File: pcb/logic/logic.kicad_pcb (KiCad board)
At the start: 4 copper layers, 40.5 x 65 mm, 10 parts, among them J1 Conn_02x02_Odd_Even, J2 Conn_02x03_Odd_Even, J3 Conn_02x02_Odd_Even, J4 Conn_02x03_Odd_Even, J5 Conn_02x02_Odd_Even, J6 Conn_02x03_Odd_Even, U4 STM32G431C6Tx

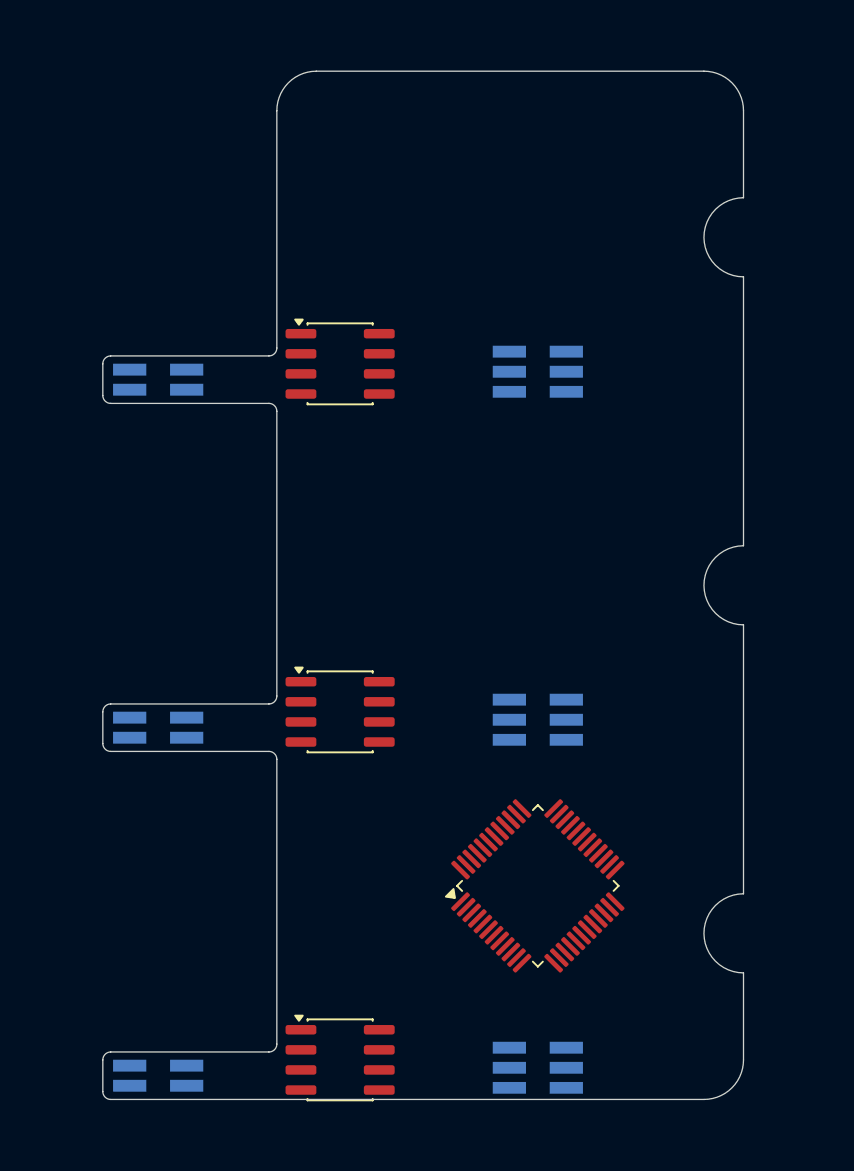
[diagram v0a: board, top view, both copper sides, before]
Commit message: Finish rev 1
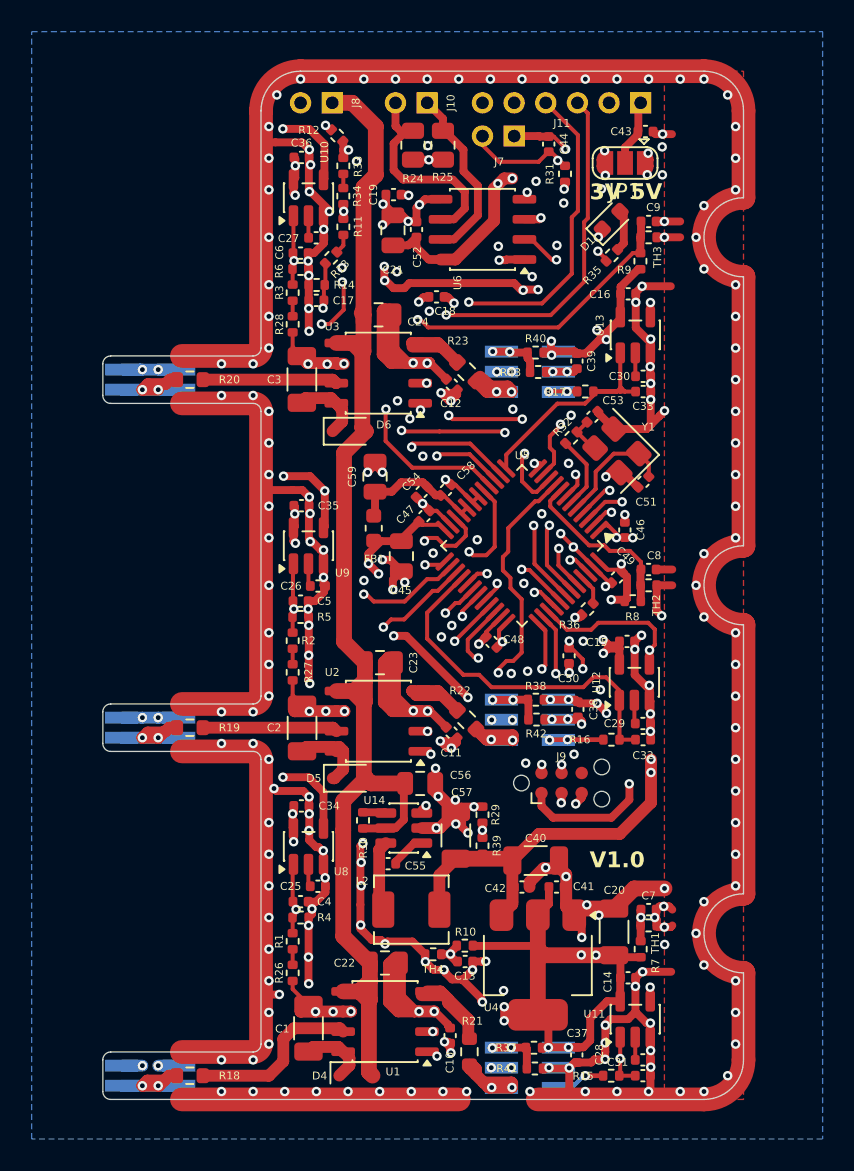
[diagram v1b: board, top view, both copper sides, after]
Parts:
- removed REF** (x3): SOIC-8_3.9x4.9mm_P1.27mm, Package_SO:SOIC-8_3.9x4.9mm_P1.27mm
- added C1: 4u7, Capacitor_SMD:C_1206_3216Metric, F.Cu at (72.5, 78.0)
- added C10: 100n, Capacitor_SMD:C_0402_1005Metric, F.Cu at (81.5, 78.5)
- added C11: 100n, Capacitor_SMD:C_0402_1005Metric, F.Cu at (81.5, 59.3)
- added C12: 100n, Capacitor_SMD:C_0402_1005Metric, F.Cu at (81.6, 37.3)
- added C13: 100n, Capacitor_SMD:C_0402_1005Metric, F.Cu at (82.4, 73.8)
- added C14: 100n, Capacitor_SMD:C_0402_1005Metric, F.Cu at (92.7, 74.8)
- added C15: 100n, Capacitor_SMD:C_0402_1005Metric, F.Cu at (92.6, 53.5)
- added C16: 100n, Capacitor_SMD:C_0402_1005Metric, F.Cu at (92.7, 31.6)
- added C17: 220p, Capacitor_SMD:C_0402_1005Metric, F.Cu at (73.0, 32.0)
- added C18: 10n, Capacitor_SMD:C_0402_1005Metric, F.Cu at (80.6, 31.8)
- added C19: 100n, Capacitor_SMD:C_0402_1005Metric, F.Cu at (77.9, 25.3)
- added C2: 4u7, Capacitor_SMD:C_1206_3216Metric, F.Cu at (72.1, 59.0)
- added C20: 22u, Capacitor_SMD:C_1206_3216Metric, F.Cu at (91.8, 71.9)
- added C21: 4u7, Capacitor_SMD:C_0805_2012Metric, F.Cu at (77.8, 27.6)
- added C22: 4u7, Capacitor_SMD:C_0805_2012Metric, F.Cu at (77.3, 73.9)
- added C23: 4u7, Capacitor_SMD:C_0805_2012Metric, F.Cu at (77.0, 54.9)
- added C24: 4u7, Capacitor_SMD:C_0805_2012Metric, F.Cu at (76.9, 32.9)
- added C25: 10n, Capacitor_SMD:C_0402_1005Metric, F.Cu at (73.1, 69.0)
- added C26: 10n, Capacitor_SMD:C_0402_1005Metric, F.Cu at (73.1, 50.0)
- added C27: 10n, Capacitor_SMD:C_0402_1005Metric, F.Cu at (73.0, 28.0)
- added C28: 10n, Capacitor_SMD:C_0402_1005Metric, F.Cu at (93.6, 80.0)
- added C29: 10n, Capacitor_SMD:C_0402_1005Metric, F.Cu at (93.6, 58.7)
- added C3: 4u7, Capacitor_SMD:C_1206_3216Metric, F.Cu at (72.1, 37.0)
- added C30: 10n, Capacitor_SMD:C_0402_1005Metric, F.Cu at (93.7, 36.8)
- added C31: 1n, Capacitor_SMD:C_0402_1005Metric, F.Cu at (93.6, 81.0)
- added C32: 1n, Capacitor_SMD:C_0402_1005Metric, F.Cu at (93.7, 59.8)
- added C33: 1n, Capacitor_SMD:C_0402_1005Metric, F.Cu at (93.7, 37.8)
- added C34: 100n, Capacitor_SMD:C_0402_1005Metric, F.Cu at (72.1, 63.9)
- added C35: 100n, Capacitor_SMD:C_0402_1005Metric, F.Cu at (72.1, 45.0)
- added C36: 100n, Capacitor_SMD:C_0402_1005Metric, F.Cu at (72.1, 23.0)
- added C37: 100n, Capacitor_SMD:C_0402_1005Metric, F.Cu at (89.5, 79.7)
- added C38: 100n, Capacitor_SMD:C_0402_1005Metric, F.Cu at (89.5, 57.8)
- added C39: 100n, Capacitor_SMD:C_0402_1005Metric, F.Cu at (89.5, 35.8)
- added C4: 220p, Capacitor_SMD:C_0402_1005Metric, F.Cu at (72.0, 70.0)
- added C40: 22u, Capacitor_SMD:C_1206_3216Metric, F.Cu at (86.9, 67.4)
- added C41: 100n, Capacitor_SMD:C_0402_1005Metric, F.Cu at (88.2, 69.1)
- added C42: 100n, Capacitor_SMD:C_0402_1005Metric, F.Cu at (86.0, 69.1)
- added C43: 100n, Capacitor_SMD:C_0402_1005Metric, F.Cu at (93.8, 21.3)
- added C44: 100n, Capacitor_SMD:C_0402_1005Metric, F.Cu at (87.7, 22.1)
- added C45: 4u7, Capacitor_SMD:C_0805_2012Metric, F.Cu at (78.4, 48.2)
- added C46: 100n, Capacitor_SMD:C_0402_1005Metric, F.Cu at (92.5, 46.5)
- added C47: 100n, Capacitor_SMD:C_0402_1005Metric, F.Cu at (79.8, 45.6)
- added C48: 100n, Capacitor_SMD:C_0402_1005Metric, F.Cu at (84.1, 53.6)
- added C49: 100n, Capacitor_SMD:C_0402_1005Metric, F.Cu at (92.0, 49.5)
- added C5: 220p, Capacitor_SMD:C_0402_1005Metric, F.Cu at (72.0, 51.0)
- added C50: 100n, Capacitor_SMD:C_0402_1005Metric, F.Cu at (89.0, 54.5)
- added C51: 10p, Capacitor_SMD:C_0402_1005Metric, F.Cu at (93.7, 43.5)
- added C52: 100n, Capacitor_SMD:C_0402_1005Metric, F.Cu at (79.3, 27.5)
- added C53: 10p, Capacitor_SMD:C_0402_1005Metric, F.Cu at (90.5, 39.3)
- added C54: 100n, Capacitor_SMD:C_0402_1005Metric, F.Cu at (79.7, 44.1)
- added C55: 100n, Capacitor_SMD:C_0402_1005Metric, F.Cu at (77.5, 67.6)
- added C56: 4u7, Capacitor_SMD:C_0805_2012Metric, F.Cu at (79.6, 62.5)
- added C57: 22u, Capacitor_SMD:C_1206_3216Metric, F.Cu at (81.8, 65.8)
- added C58: 1n, Capacitor_SMD:C_0402_1005Metric, F.Cu at (81.2, 44.0)
- added C59: 4u7, Capacitor_SMD:C_0805_2012Metric, F.Cu at (76.7, 43.1)
- added C6: 220p, Capacitor_SMD:C_0402_1005Metric, F.Cu at (72.0, 29.0)
- added C7: 100n, Capacitor_SMD:C_0402_1005Metric, F.Cu at (94.0, 70.5)
- added C8: 100n, Capacitor_SMD:C_0402_1005Metric, F.Cu at (94.0, 49.0)
- added C9: 100n, Capacitor_SMD:C_0402_1005Metric, F.Cu at (94.0, 27.0)
- added D1: LED, LED_SMD:LED_0603_1608Metric, F.Cu at (91.6, 26.9)
- added D4: 1N4148WS, Diode_SMD:D_SOD-323, F.Cu at (75.5, 81.0)
- added D5: 1N4148WS, Diode_SMD:D_SOD-323, F.Cu at (75.1, 62.2)
- added D6: 1N4148WS, Diode_SMD:D_SOD-323, F.Cu at (75.1, 40.3)
- added FB1: 120, Inductor_SMD:L_0603_1608Metric, F.Cu at (76.6, 46.4)
- added G1: LOGO, LOGO, B.Cu at (82.3, 47.1)
- added G2: LOGO, LOGO, B.Cu at (85.2, 68.5)
- added G3: LOGO, LOGO, B.Cu at (74.3, 74.7)
- added G4: LOGO, LOGO, B.Cu at (78.2, 30.3)
- added G5: LOGO, LOGO, B.Cu at (75.8, 58.9)
- added J10: Conn_01x02, User_Footprints:1x02_2.00mm_Solder, B.Cu at (80.0, 19.5)
- added J11: Conn_01x06, User_Footprints:1x06_2.00mm_Solder, B.Cu at (93.5, 19.5)
- added J7: Conn_01x02, User_Footprints:1x02_2.00mm_Solder, B.Cu at (85.5, 21.6)
- added J8: Conn_01x02, User_Footprints:1x02_2.00mm_Solder, B.Cu at (74.0, 19.5)
- added J9: Conn_ARM_SWD_TagConnect_TC2030-NL, Connector:Tag-Connect_TC2030-IDC-NL_2x03_P1.27mm_Vertical, F.Cu at (88.5, 62.5)
- added JP1: SolderJumper_3_Open, Jumper:SolderJumper-3_P1.3mm_Open_RoundedPad1.0x1.5mm, F.Cu at (92.5, 23.3)
- added L2: 4u7, Inductor_SMD:L_TechFuse_SL0420, F.Cu at (79.0, 70.5)
- added R1: 33k, Resistor_SMD:R_0402_1005Metric, F.Cu at (71.5, 72.5)
- added R10: 2k2, Resistor_SMD:R_0402_1005Metric, F.Cu at (82.4, 72.8)
- added R11: 33k, Resistor_SMD:R_0402_1005Metric, F.Cu at (74.7, 27.3)
- added R12: 2k2, Resistor_SMD:R_0402_1005Metric, F.Cu at (74.3, 21.6)
- added R13: 33k, Resistor_SMD:R_0402_1005Metric, F.Cu at (73.9, 29.3)
- added R14: 2k2, Resistor_SMD:R_0402_1005Metric, F.Cu at (73.0, 31.0)
- added R15: 2k2, Resistor_SMD:R_0402_1005Metric, F.Cu at (91.6, 81.0)
- added R16: 2k2, Resistor_SMD:R_0402_1005Metric, F.Cu at (91.7, 59.8)
- added R17: 2k2, Resistor_SMD:R_0402_1005Metric, F.Cu at (90.0, 37.7)
- added R18: 1, Resistor_SMD:R_0603_1608Metric, F.Cu at (65.0, 81.0)
- added R19: 1, Resistor_SMD:R_0603_1608Metric, F.Cu at (65.0, 59.0)
- added R2: 33k, Resistor_SMD:R_0402_1005Metric, F.Cu at (71.5, 53.5)
- added R20: 1, Resistor_SMD:R_0603_1608Metric, F.Cu at (65.0, 37.0)
- added R21: 1, Resistor_SMD:R_0603_1608Metric, F.Cu at (82.7, 79.5)
- added R22: 1, Resistor_SMD:R_0603_1608Metric, F.Cu at (82.5, 58.5)
- added R23: 1, Resistor_SMD:R_0603_1608Metric, F.Cu at (82.5, 36.5)
- added R24: 51, Resistor_SMD:R_0805_2012Metric, F.Cu at (79.1, 22.2)
- added R25: 51, Resistor_SMD:R_0805_2012Metric, F.Cu at (81.0, 22.2)
- added R26: 33k, Resistor_SMD:R_0402_1005Metric, F.Cu at (71.5, 74.5)
- added R27: 33k, Resistor_SMD:R_0402_1005Metric, F.Cu at (71.5, 55.5)
- added R28: 33k, Resistor_SMD:R_0402_1005Metric, F.Cu at (71.5, 33.5)
- added R29: 2k2, Resistor_SMD:R_0402_1005Metric, F.Cu at (83.5, 64.5)
- added R3: 33k, Resistor_SMD:R_0402_1005Metric, F.Cu at (71.5, 31.5)
- added R30: 33k, Resistor_SMD:R_0402_1005Metric, F.Cu at (75.9, 64.9)
- added R31: 2k2, Resistor_SMD:R_0402_1005Metric, F.Cu at (88.7, 24.0)
- added R32: 330, Resistor_SMD:R_0402_1005Metric, F.Cu at (89.1, 40.7)
- added R33: 33k, Resistor_SMD:R_0402_1005Metric, F.Cu at (74.7, 23.5)
- added R34: 33k, Resistor_SMD:R_0402_1005Metric, F.Cu at (74.7, 25.4)
- added R35: 2k2, Resistor_SMD:R_0402_1005Metric, F.Cu at (91.7, 29.1)
- added R36: 2k2, Resistor_SMD:R_0402_1005Metric, F.Cu at (90.1, 51.5)
- added R37: 2k2, Resistor_SMD:R_0402_1005Metric, F.Cu at (86.8, 79.2)
- added R38: 2k2, Resistor_SMD:R_0402_1005Metric, F.Cu at (86.9, 57.2)
- added R39: 12k, Resistor_SMD:R_0402_1005Metric, F.Cu at (83.5, 66.5)
- added R4: 2k2, Resistor_SMD:R_0402_1005Metric, F.Cu at (72.0, 71.0)
- added R40: 2k2, Resistor_SMD:R_0402_1005Metric, F.Cu at (86.9, 35.3)
- added R41: 2k2, Resistor_SMD:R_0402_1005Metric, F.Cu at (86.8, 80.5)
- added R42: 2k2, Resistor_SMD:R_0402_1005Metric, F.Cu at (86.9, 58.5)
- added R43: 2k2, Resistor_SMD:R_0402_1005Metric, F.Cu at (87.0, 36.5)
- added R5: 2k2, Resistor_SMD:R_0402_1005Metric, F.Cu at (72.0, 52.0)
- added R6: 2k2, Resistor_SMD:R_0402_1005Metric, F.Cu at (72.0, 30.0)
- added R7: 2k2, Resistor_SMD:R_0402_1005Metric, F.Cu at (93.5, 73.0)
- added R8: 2k2, Resistor_SMD:R_0402_1005Metric, F.Cu at (93.0, 51.0)
- added R9: 2k2, Resistor_SMD:R_0402_1005Metric, F.Cu at (93.5, 29.5)
- added TH1: 10k, Resistor_SMD:R_0402_1005Metric, F.Cu at (94.0, 71.5)
- added TH2: 10k, Resistor_SMD:R_0402_1005Metric, F.Cu at (94.0, 50.0)
- added TH3: 10k, Resistor_SMD:R_0402_1005Metric, F.Cu at (94.0, 28.0)
- added TH4: 10k, Resistor_SMD:R_0402_1005Metric, F.Cu at (80.4, 73.3)
- added U1: IRS2181STR, Package_SO:JEITA_SOIC-8_3.9x4.9mm_P1.27mm, F.Cu at (77.3, 77.6)
- added U10: 74LVC1G66, Package_TO_SOT_SMD:SOT-23-5, F.Cu at (72.5, 25.5)
- added U11: 74LVC1G66, Package_TO_SOT_SMD:SOT-23-5, F.Cu at (93.2, 77.4)
- added U12: 74LVC1G66, Package_TO_SOT_SMD:SOT-23-5, F.Cu at (93.1, 56.1)
- added U13: 74LVC1G66, Package_TO_SOT_SMD:SOT-23-5, F.Cu at (93.2, 34.2)
- added U14: JW5017S, Package_TO_SOT_SMD:SOT-23-6, F.Cu at (78.5, 65.3)
- added U2: IRS2181STR, Package_SO:JEITA_SOIC-8_3.9x4.9mm_P1.27mm, F.Cu at (76.9, 58.6)
- added U3: IRS2181STR, Package_SO:JEITA_SOIC-8_3.9x4.9mm_P1.27mm, F.Cu at (76.9, 36.6)
- added U5: STM32G473CBTx, Package_QFP:LQFP-48_7x7mm_P0.5mm, F.Cu at (86.0, 47.5)
- added U6: SP485E, Package_SO:JEITA_SOIC-8_3.9x4.9mm_P1.27mm, F.Cu at (83.5, 27.5)
- added U8: 74LVC1G66, Package_TO_SOT_SMD:SOT-23-5, F.Cu at (72.5, 66.5)
- added U9: 74LVC1G66, Package_TO_SOT_SMD:SOT-23-5, F.Cu at (72.5, 47.5)
- added Y1: 16MHz, Crystal:Crystal_SMD_3225-4Pin_3.2x2.5mm, F.Cu at (92.0, 41.5)
- U4: value STM32G431C6Tx -> AMS1117-3.3; footprint Package_QFP:LQFP-48_7x7mm_P0.5mm -> Package_TO_SOT_SMD:SOT-223-3_TabPin2
- moved J4 22.0 mm to (86.5, 58.5)
- moved J6 22.0 mm to (86.5, 36.5)
- moved U4 5.00 mm to (87.0, 74.0), turned to -90 degrees
- moved J1 0.50 mm to (62.5, 81.0)
- moved J2 0.50 mm to (86.5, 80.5)
- moved J3 0.50 mm to (62.5, 59.0)
- moved J5 0.50 mm to (62.5, 37.0)
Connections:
- J1 pad 1: unconnected-(J1-Pin_1-Pad1) -> /Phase1/PH
- J1 pad 2: unconnected-(J1-Pin_2-Pad2) -> /Phase1/PH
- J1 pad 3: unconnected-(J1-Pin_3-Pad3) -> /Phase1/GH
- J1 pad 4: unconnected-(J1-Pin_4-Pad4) -> /Phase1/GH
- J2 pad 1: unconnected-(J2-Pin_1-Pad1) -> /Phase1/VREF
- J2 pad 2: unconnected-(J2-Pin_2-Pad2) -> +3V3
- J2 pad 3: unconnected-(J2-Pin_3-Pad3) -> /Phase1/SH
- J2 pad 4: unconnected-(J2-Pin_4-Pad4) -> GND
- J2 pad 5: unconnected-(J2-Pin_5-Pad5) -> /Phase1/GL
- J2 pad 6: unconnected-(J2-Pin_6-Pad6) -> /Phase1/CR
- J3 pad 1: unconnected-(J3-Pin_1-Pad1) -> /Phase2/PH
- J3 pad 2: unconnected-(J3-Pin_2-Pad2) -> /Phase2/PH
- J3 pad 3: unconnected-(J3-Pin_3-Pad3) -> /Phase2/GH
- J3 pad 4: unconnected-(J3-Pin_4-Pad4) -> /Phase2/GH
- J4 pad 1: unconnected-(J4-Pin_1-Pad1) -> /Phase2/VREF
- J4 pad 2: unconnected-(J4-Pin_2-Pad2) -> +3V3
- J4 pad 3: unconnected-(J4-Pin_3-Pad3) -> /Phase2/SH
- J4 pad 4: unconnected-(J4-Pin_4-Pad4) -> GND
- J4 pad 5: unconnected-(J4-Pin_5-Pad5) -> /Phase2/GL
- J4 pad 6: unconnected-(J4-Pin_6-Pad6) -> /Phase2/CR
- J5 pad 1: unconnected-(J5-Pin_1-Pad1) -> /Phase3/PH
- J5 pad 2: unconnected-(J5-Pin_2-Pad2) -> /Phase3/PH
- J5 pad 3: unconnected-(J5-Pin_3-Pad3) -> /Phase3/GH
- J5 pad 4: unconnected-(J5-Pin_4-Pad4) -> /Phase3/GH
- J6 pad 1: unconnected-(J6-Pin_1-Pad1) -> /Phase3/VREF
- J6 pad 2: unconnected-(J6-Pin_2-Pad2) -> +3V3
- J6 pad 3: unconnected-(J6-Pin_3-Pad3) -> /Phase3/SH
- J6 pad 4: unconnected-(J6-Pin_4-Pad4) -> GND
- J6 pad 5: unconnected-(J6-Pin_5-Pad5) -> /Phase3/GL
- J6 pad 6: unconnected-(J6-Pin_6-Pad6) -> /Phase3/CR
- U4 pad 1: unconnected-(U4-VBAT-Pad1) -> GND
- U4 pad 2: unconnected-(U4-PC13-Pad2) -> +3V3
- U4 pad 3: unconnected-(U4-PC14-Pad3) -> +5V
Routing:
- net +3V3: track 0.00 -> 251.2 mm, vias 0 -> 37
- net GND: track 0.00 -> 207.4 mm, vias 0 -> 254
- net +5V: track 0.00 -> 92.7 mm, vias 0 -> 6
- net +15V: track 0.00 -> 82.2 mm
- net /FLTV: track 0.00 -> 71.1 mm, vias 0 -> 5
- net /QZ: track 0.00 -> 63.9 mm, vias 0 -> 3
- net /FLTC: track 0.00 -> 58.1 mm, vias 0 -> 3
- net /TEMP: track 0.00 -> 49.6 mm, vias 0 -> 2
- net /ACUR: track 0.00 -> 49.0 mm, vias 0 -> 2
- net /ATEMP: track 0.00 -> 45.5 mm, vias 0 -> 2
- net /QA: track 0.00 -> 42.8 mm, vias 0 -> 2
- net /QB: track 0.00 -> 40.7 mm, vias 0 -> 2
- net /BUSL: track 0.00 -> 39.1 mm, vias 0 -> 5
- net /AINH: track 0.00 -> 35.4 mm, vias 0 -> 2
- net /CTEMP: track 0.00 -> 34.5 mm, vias 0 -> 2
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- added copper zone on B.Cu, net GND
- added copper zone on F.Cu, net GND
- added copper zone on In1.Cu, net GND
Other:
- outline, holes or cut-outs redrawn
- board text added: "15V"
- board text added: "3V"
- board text added: "5V"
- board text added: "A"
- board text added: "B"
- board text added: "GND"
- board text added: "MT"
- board text added: "Miguel Flores-Acton"
- board text added: "No Inve rter?"
- board text added: "RSA"
- board text added: "RSB"
- board text added: "Soap Inverter Logic Board V1.0"
- board text added: "V1.0"
- board text added: "VBUS"
- board text added: "VCC"
- board text added: "Z"
- board text added: "me when rust"
